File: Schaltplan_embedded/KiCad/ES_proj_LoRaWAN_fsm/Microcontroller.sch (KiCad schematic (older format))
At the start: 16 parts, among them J1 Conn_02x05_Odd_Even, J2 Conn_01x02, U1 STM32L476RGTx, Y1 Crystal 8Mhz

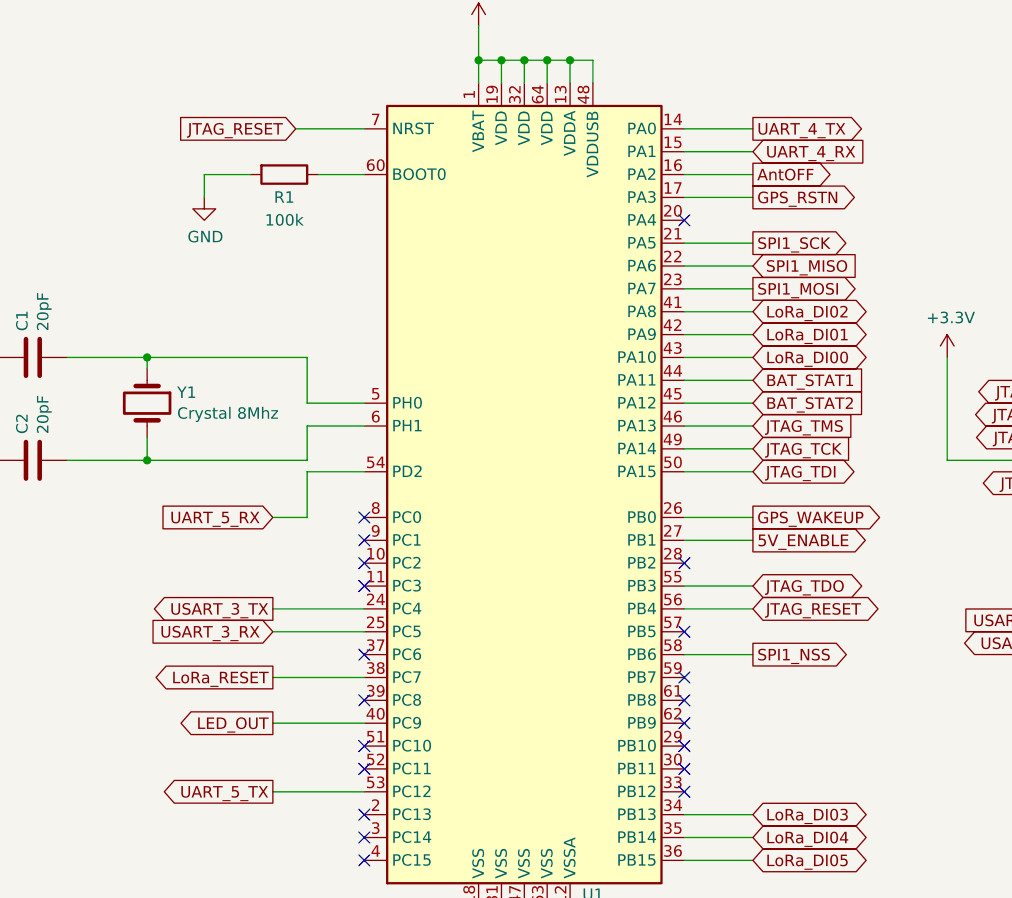
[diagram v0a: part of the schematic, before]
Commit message: Neue platine
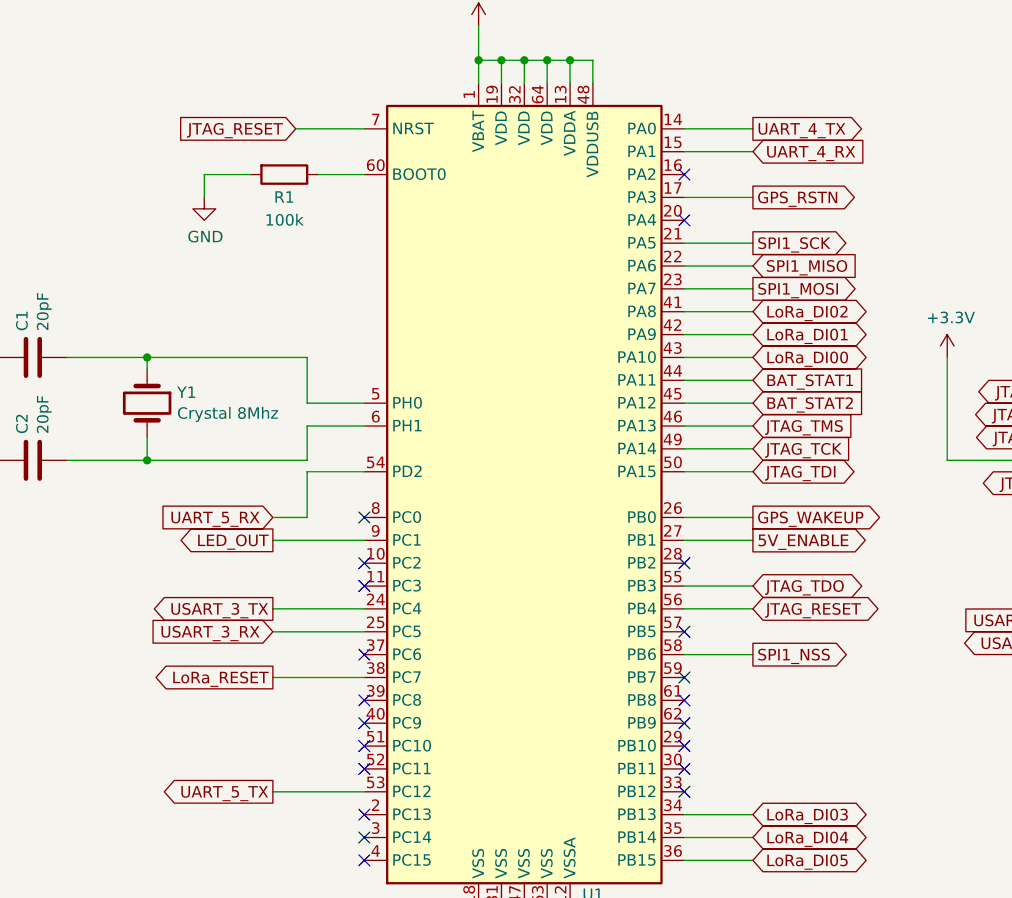
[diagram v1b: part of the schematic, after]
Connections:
- net LED_OUT: now also U1.9 (PC1); no longer U1.40 (PC9)
- net AntOFF: no longer names the net of U1.16 (PA2)
- no-connect marks 22 -> 23
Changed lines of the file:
@@
 Wire Wire Line
 	2700 3250 2700 3350
-Text GLabel 3000 5650 0    50   Output ~ 0
+Text GLabel 3000 4850 0    50   Output ~ 0
 LED_OUT
 Text GLabel 8600 4350 0    50   Input ~ 0
@@
 NoConn ~ 3400 5050
 NoConn ~ 3400 4950
-NoConn ~ 3400 4850
 NoConn ~ 3400 4750
 NoConn ~ 4800 4950
@@
 	4400 2750 4400 2850
 Connection ~ 4300 2750
-Text GLabel 5100 3250 2    50   Output ~ 0
-AntOFF
 $Comp
 L power:+3.3V #PWR03
@@
 Wire Wire Line
 	4800 3850 5100 3850
-Wire Wire Line
-	3000 5650 3400 5650
 $Comp
 L MCU_ST_STM32L4:STM32L476RGTx U1
@@
 NoConn ~ 4800 5850
 NoConn ~ 4800 5950
-Wire Wire Line
-	4800 3250 5100 3250
 NoConn ~ 4800 5550
+Wire Wire Line
+	3400 4850 3000 4850
+NoConn ~ 3400 5650
+NoConn ~ 4800 3250
 $EndSCHEMATC
